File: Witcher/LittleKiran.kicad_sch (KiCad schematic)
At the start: 18 parts, among them J1 XT60PW-M, J2 XT60PW-M, J3 XT60PW-F, Q1 PXP012-30QLJ, Q2 PXP012-30QLJ, Q3 PXP012-30QLJ, Q4 FDN340P, U1 LTC4412xS6, U2 LTC4412xS6

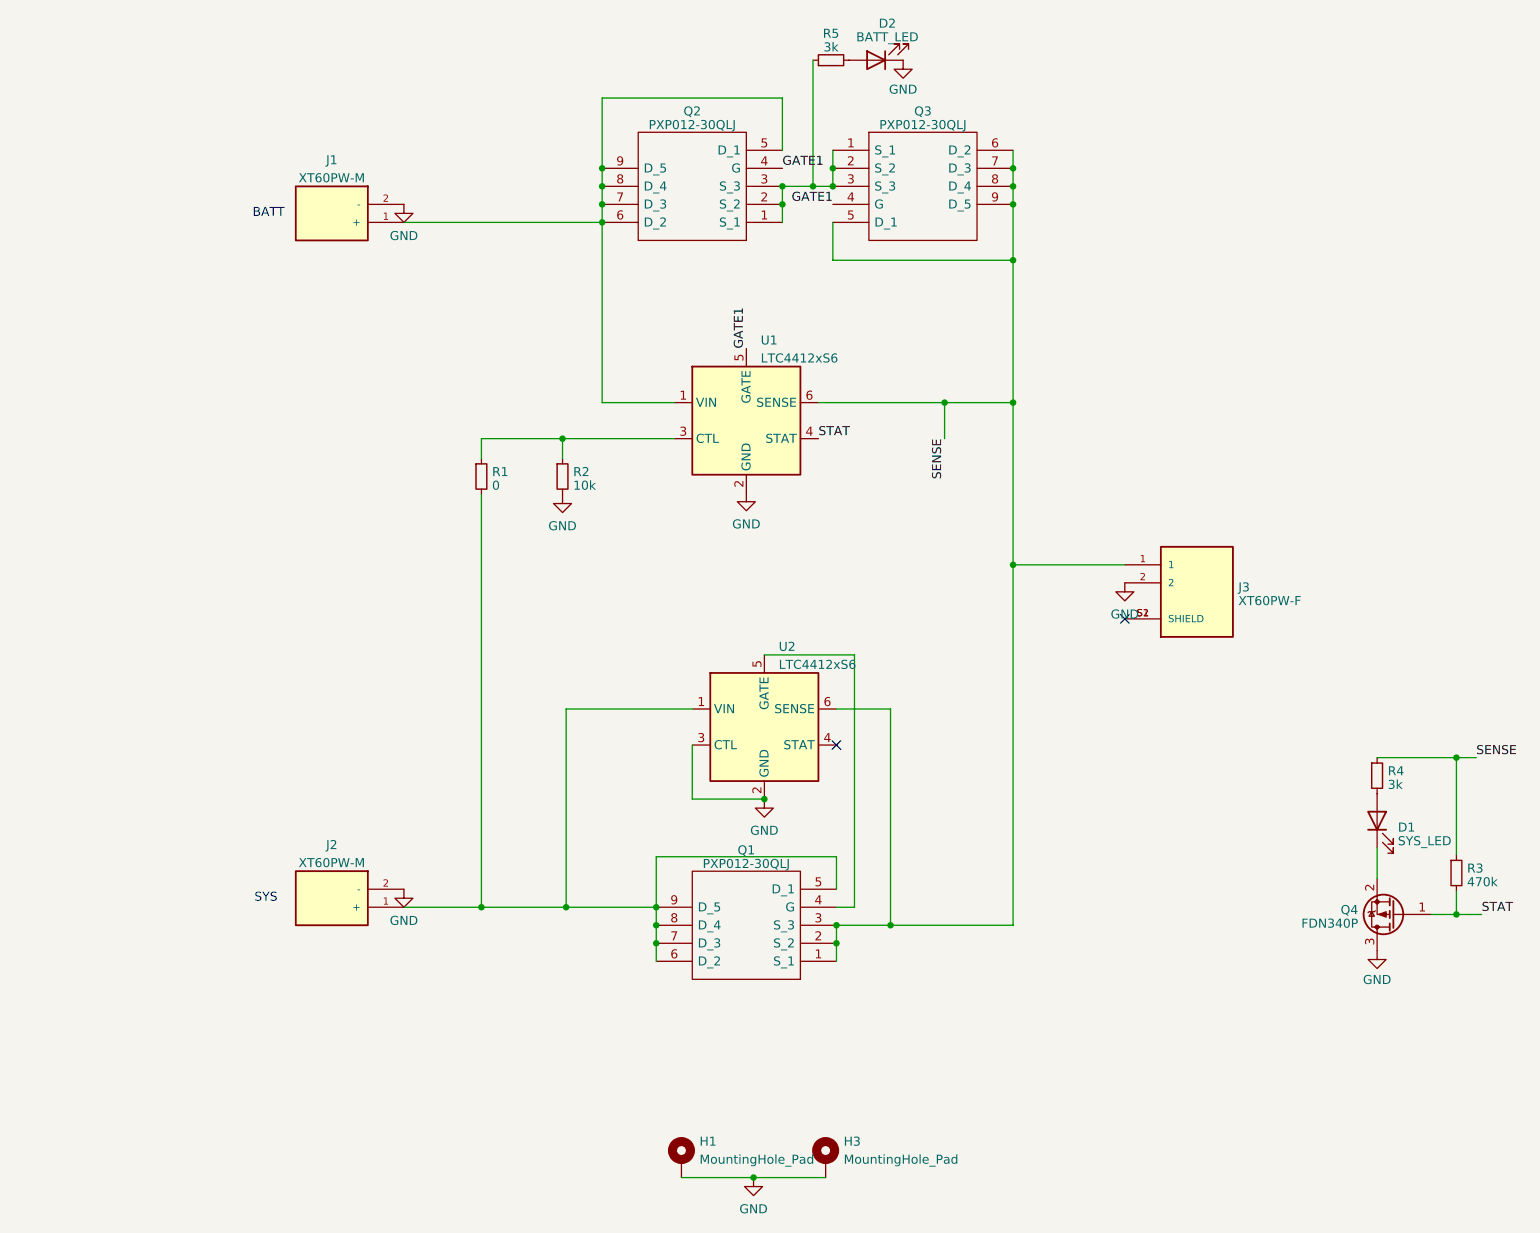
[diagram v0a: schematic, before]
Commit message: fixes
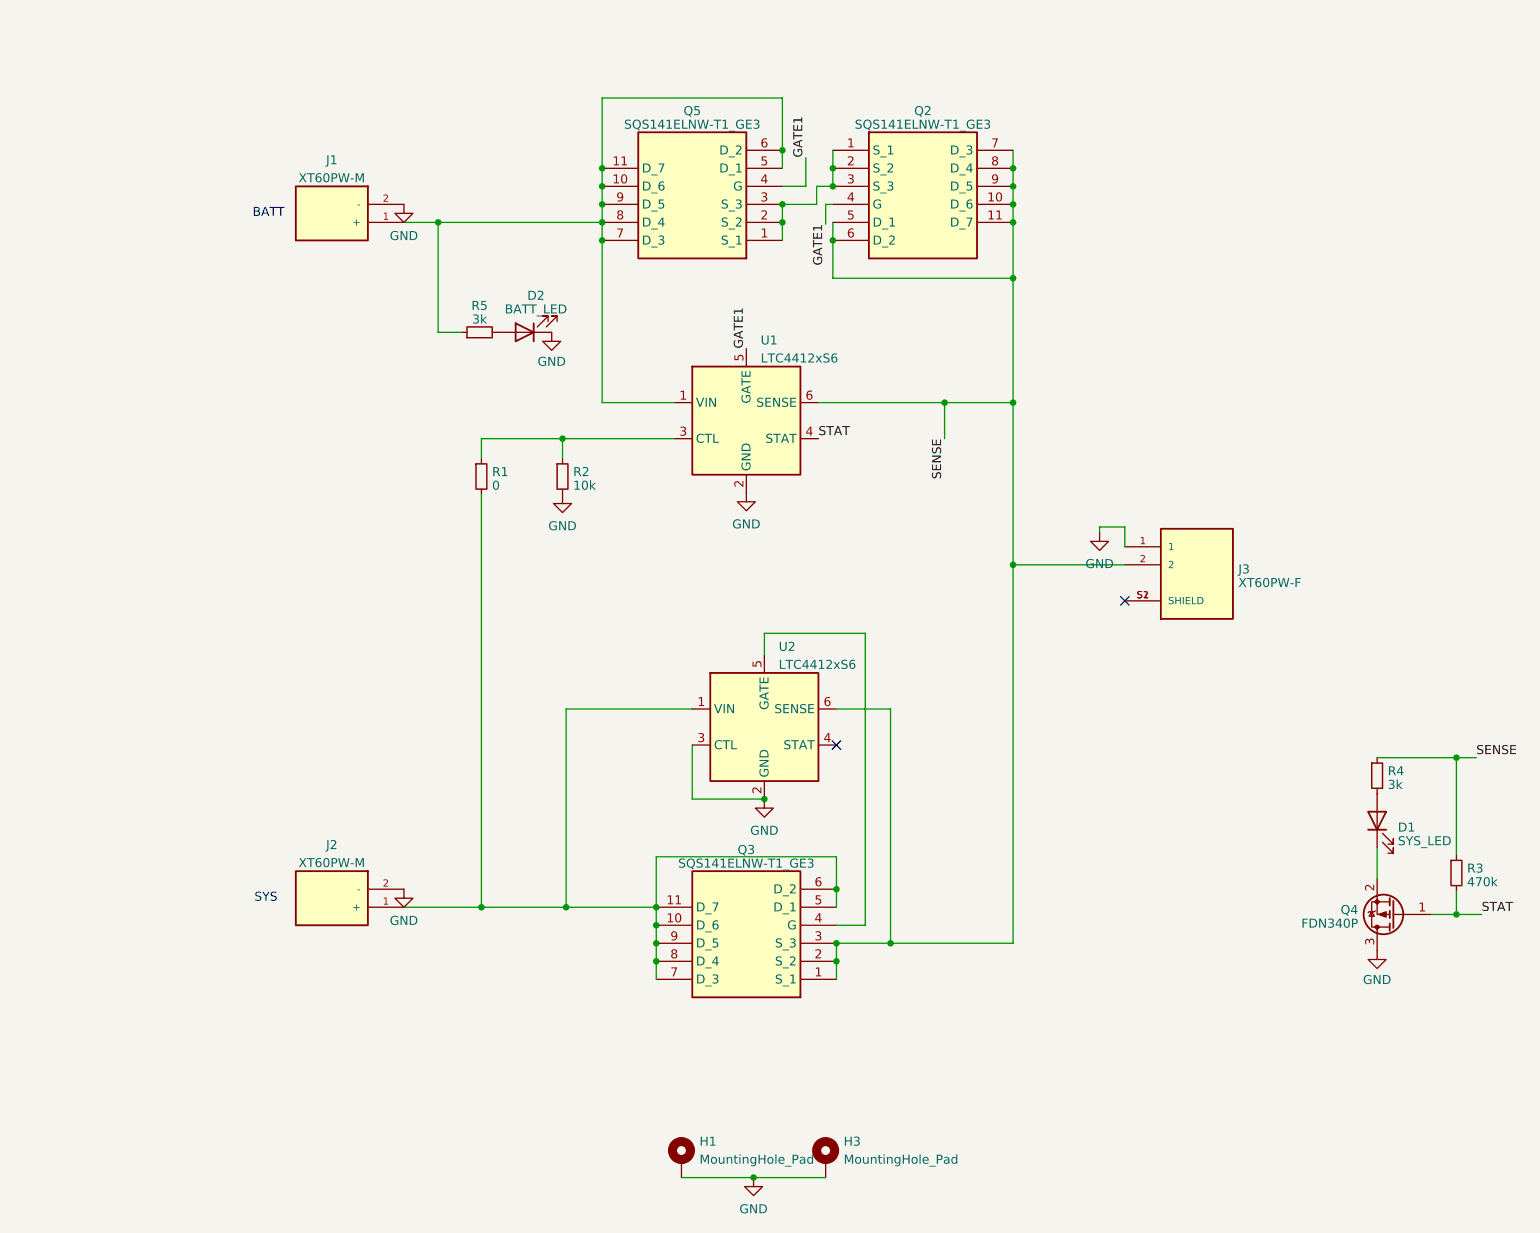
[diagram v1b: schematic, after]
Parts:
- removed Q1, Q2, Q3: PXP012-30QLJ, iclr:PXP01230QLJ, symbol iclr:PXP012-30QLJ
- added Q2, Q3, Q5: SQS141ELNW-T1_GE3, SQS850ENT1_GE3, symbol iclr:SQS141ELNW-T1_GE3
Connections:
- net GATE1: now also Q2.4 (G), Q5.4 (G)
- net GND: now also J3.1; no longer J3.2
- net SENSE: now also J3.2, Q2.10 (D_6), Q2.11 (D_7), Q2.5 (D_1), Q2.6 (D_2), Q2.7 (D_3), Q2.8 (D_4), Q2.9 (D_5), Q3.1 (S_1), Q3.2 (S_2), Q3.3 (S_3); no longer J3.1
- net at J2.1 (+), R1.2, U2.1 (VIN): now also Q3.10 (D_6), Q3.11 (D_7), Q3.5 (D_1), Q3.6 (D_2), Q3.7 (D_3), Q3.8 (D_4), Q3.9 (D_5)
- net at U2.5 (GATE): now also Q3.4 (G)
- net at R5.1: now also J1.1 (+), U1.1 (VIN), Q5.10 (D_6), Q5.11 (D_7), Q5.5 (D_1), Q5.6 (D_2), Q5.7 (D_3), Q5.8 (D_4), Q5.9 (D_5)
- new net: Q2.1 (S_1), Q2.2 (S_2), Q2.3 (S_3), Q5.1 (S_1), Q5.2 (S_2), Q5.3 (S_3)
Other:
- moved on the sheet: D2, J3, R5

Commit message: v2.0
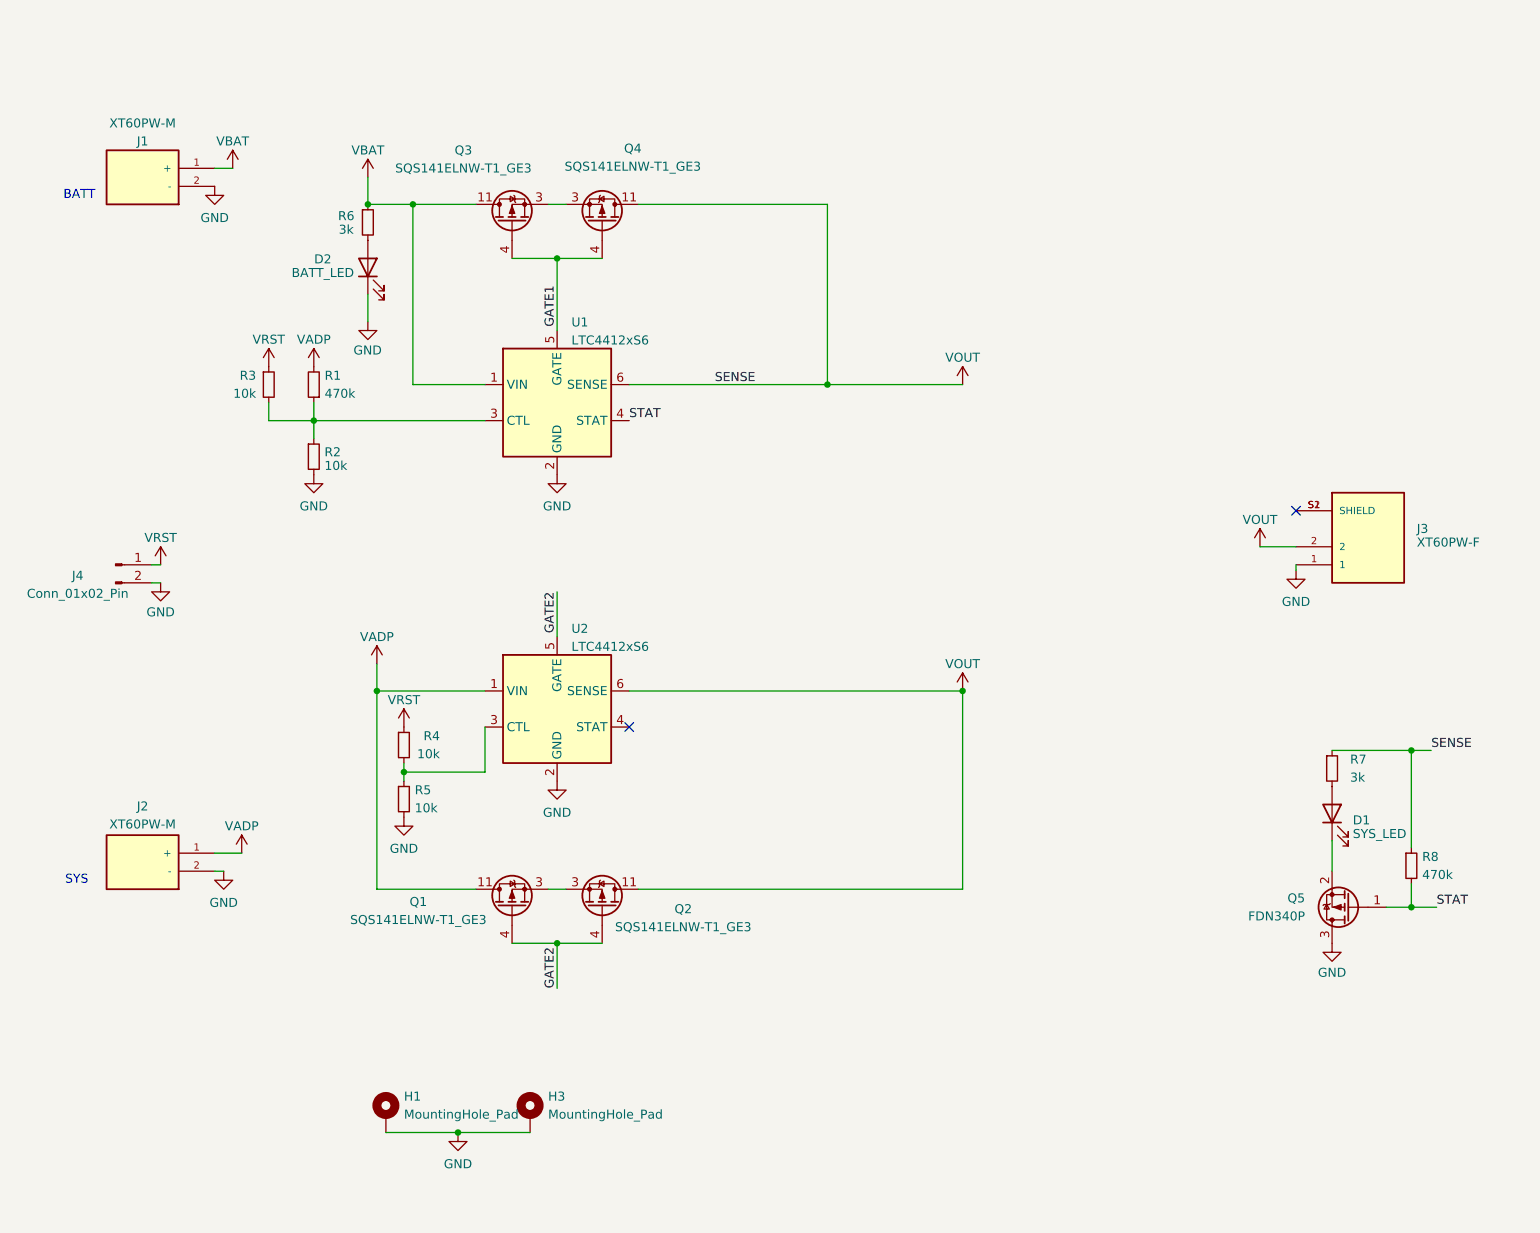
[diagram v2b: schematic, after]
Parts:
- removed Q5: SQS141ELNW-T1_GE3, SQS850ENT1_GE3, symbol iclr:SQS141ELNW-T1_GE3
- added J4: Conn_01x02_Pin, Connector_Molex:Molex_Nano-Fit_105313-xx02_1x02_P2.50mm_Horizontal, symbol Connector:Conn_01x02_Pin
- added Q2, Q3: SQS141ELNW-T1_GE3, iclr:SQS850ENT1_GE3, symbol iclr:SQS141ELNW-T1_GE3
- added R3, R4, R5: 10k, Resistor_SMD:R_0402_1005Metric, symbol Device:R_Small
- Q1: renamed from Q3; footprint SQS850ENT1_GE3 -> iclr:SQS850ENT1_GE3
- Q4: renamed from Q2; footprint SQS850ENT1_GE3 -> iclr:SQS850ENT1_GE3
- R1: value 0 -> 470k; footprint Resistor_SMD:R_0603_1608Metric -> Resistor_SMD:R_0402_1005Metric
- R2: footprint Resistor_SMD:R_0603_1608Metric -> Resistor_SMD:R_0402_1005Metric
- renumbered Q4 to Q5, R5 to R6, R4 to R7, R3 to R8
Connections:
- net GATE1: now also Q3.4
- net GND: now also J4.2 (Pin_2), R5.2; no longer U2.3 (CTL)
- net VADP: now reaches J2.1 (+), Q1.10, Q1.11, Q1.5, Q1.6, Q1.7, Q1.8, Q1.9, R1.2, U2.1 (VIN)
- net GATE2: now reaches Q1.4, U2.5 (GATE)
- net GATE2: now also Q2.4
- net VBAT: now reaches J1.1 (+), R6.1, U1.1 (VIN)
- net VBAT: now also Q3.10, Q3.11, Q3.5, Q3.6, Q3.7, Q3.8, Q3.9
- net at R1.1, R2.1, U1.3 (CTL): now also R3.2
- net at Q4.1, Q4.2, Q4.3: now also Q3.1, Q3.2, Q3.3
- net SENSE renamed VOUT
- net VOUT: now also Q2.10, Q2.11, Q2.5, Q2.6, Q2.7, Q2.8, Q2.9; no longer Q1.1 (S_1), Q1.2 (S_2), Q1.3 (S_3)
- new net: R4.2, R5.1, U2.3 (CTL)
- new net: Q1.1, Q1.2, Q1.3, Q2.1, Q2.2, Q2.3
- new net VRST: J4.1 (Pin_1), R3.1, R4.1
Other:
- moved on the sheet: D1, D2, H1, H3, J1, J2, J3, Q5, R1, R2, R6, R7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

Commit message: my nanofit 3d model reset itself
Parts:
- J4: footprint Connector_Molex:Molex_Nano-Fit_105313-xx02_1x02_P2.50mm_Horizontal -> iclr:Molex_Nano-Fit_105313-xx02_1x02_P2.50mm_Horizontal
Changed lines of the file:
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@@
 			)
 		)
-		(property "Footprint" "Connector_Molex:Molex_Nano-Fit_105313-xx02_1x02_P2.50mm_Horizontal"
+		(property "Footprint" "iclr:Molex_Nano-Fit_105313-xx02_1x02_P2.50mm_Horizontal"
 			(at 60.96 91.44 0)
 			(effects
